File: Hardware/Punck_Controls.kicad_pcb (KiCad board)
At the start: 2 copper layers, 91.2 x 110 mm, 36 parts, among them J1 Conn_01x12_Female, J10 Kick_In, J11 USB_B_Micro, J12 Tempo_Out, J13 Audio_Out_L, J14 Audio_Out_R, J15 Midi_In, J2 Conn_01x12_Female, J3 Conn_01x12_Female, J4 Conn_01x12_Female, J5 Snare_In, J6 CH_In, J7 OH_In, J8 SamplerA_In, J9 SamplerB_In

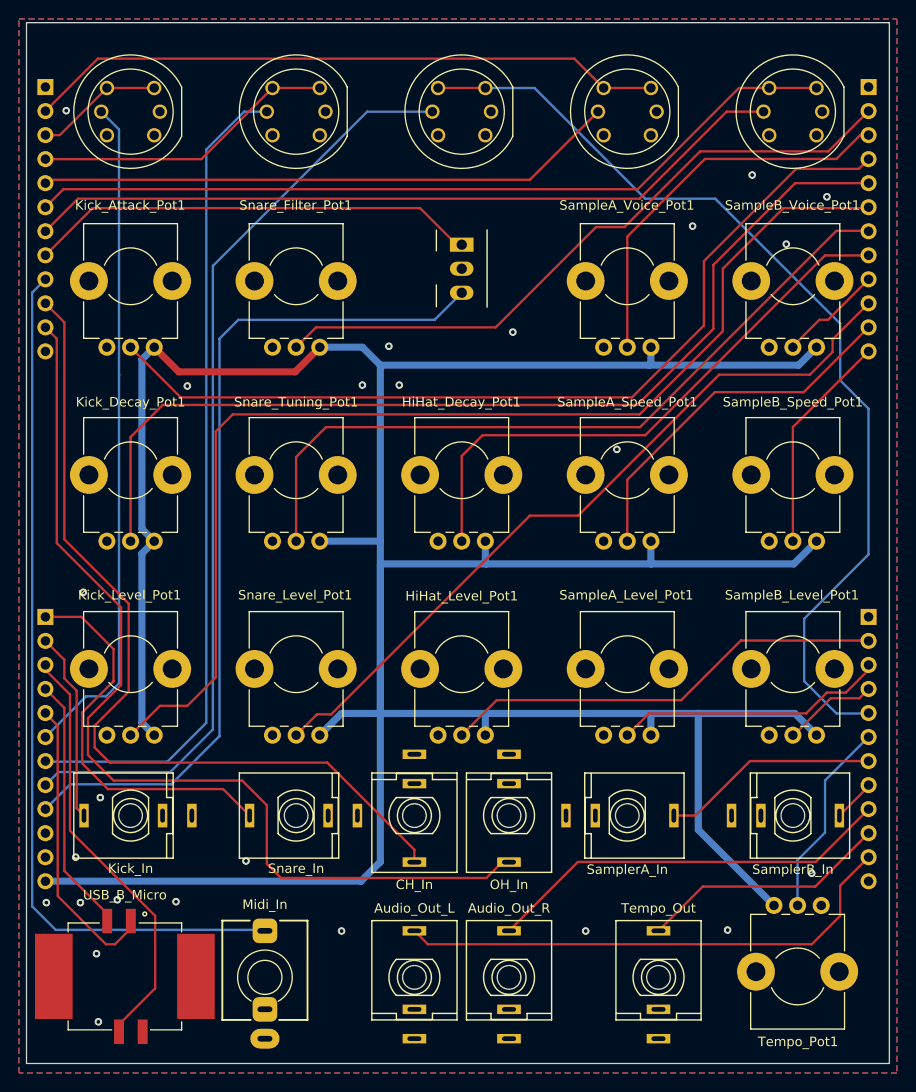
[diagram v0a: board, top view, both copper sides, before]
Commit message: Final tweaking and v1 gerber creation; JLC order placed
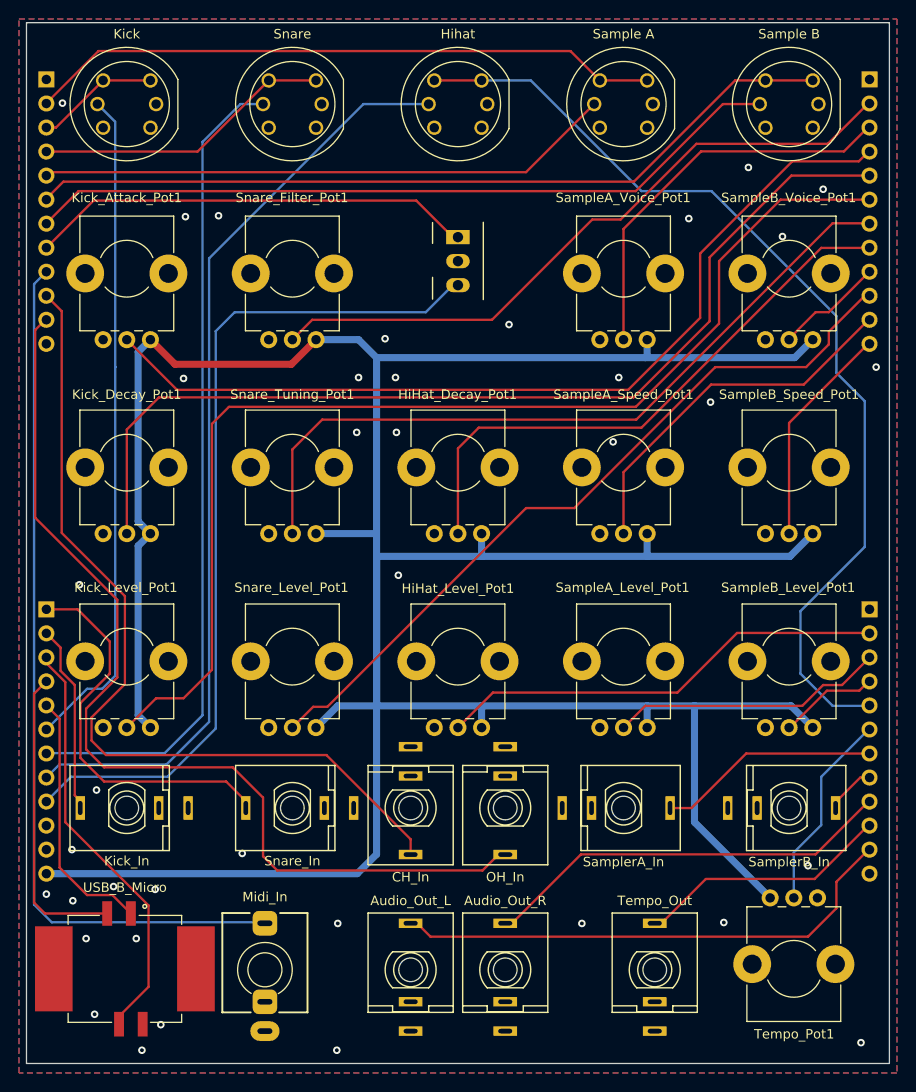
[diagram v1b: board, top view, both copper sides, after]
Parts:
- moved J10 0.89 mm to (80.6, 133.0)
- moved J12 0.89 mm to (136.4, 150.1)
- moved J13 0.89 mm to (110.6, 150.1)
- moved J14 0.89 mm to (120.6, 150.1)
- moved J5 0.89 mm to (98.1, 133.0)
- moved J6 0.89 mm to (110.6, 133.0)
- moved J7 0.89 mm to (120.6, 133.0)
- moved J8 0.89 mm to (133.1, 133.0)
- moved J9 0.89 mm to (150.6, 133.0)
- moved Tempo_Pot1 0.89 mm to (151.1, 150.0)
- moved BTN1 0.89 mm to (80.6, 58.6)
- moved BTN2 0.89 mm to (98.1, 58.6)
- moved BTN3 0.89 mm to (115.6, 58.6)
- moved BTN4 0.89 mm to (133.1, 58.6)
- moved BTN5 0.89 mm to (150.6, 58.6)
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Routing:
- net /USB_DM: track 27.2 -> 32.1 mm
- net /USB_VBUS: track 31.1 -> 27.3 mm
- net /USB_DP: track 45.9 -> 44.5 mm
- net /SAMPLER_B_IN: track 4.50 -> 5.28 mm
- net /OH_IN: track 104.2 -> 104.7 mm
- net /SN_LED: track 87.4 -> 86.9 mm
- net /HH_LED: track 99.1 -> 98.6 mm
- net /KI_BTN: track 13.6 -> 13.1 mm
- net /SN_BTN: track 32.1 -> 31.6 mm
- net GND: vias 25 -> 38
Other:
- board text added: "Hihat"
- board text added: "Kick"
- board text added: "Mountjoy Modular Punck Controls v1.0"
- board text added: "Sample A"
- board text added: "Sample B"
- board text added: "Snare"
